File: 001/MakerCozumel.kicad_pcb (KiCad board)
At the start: 2 copper layers, 60.3 x 54.2 mm, 5 parts

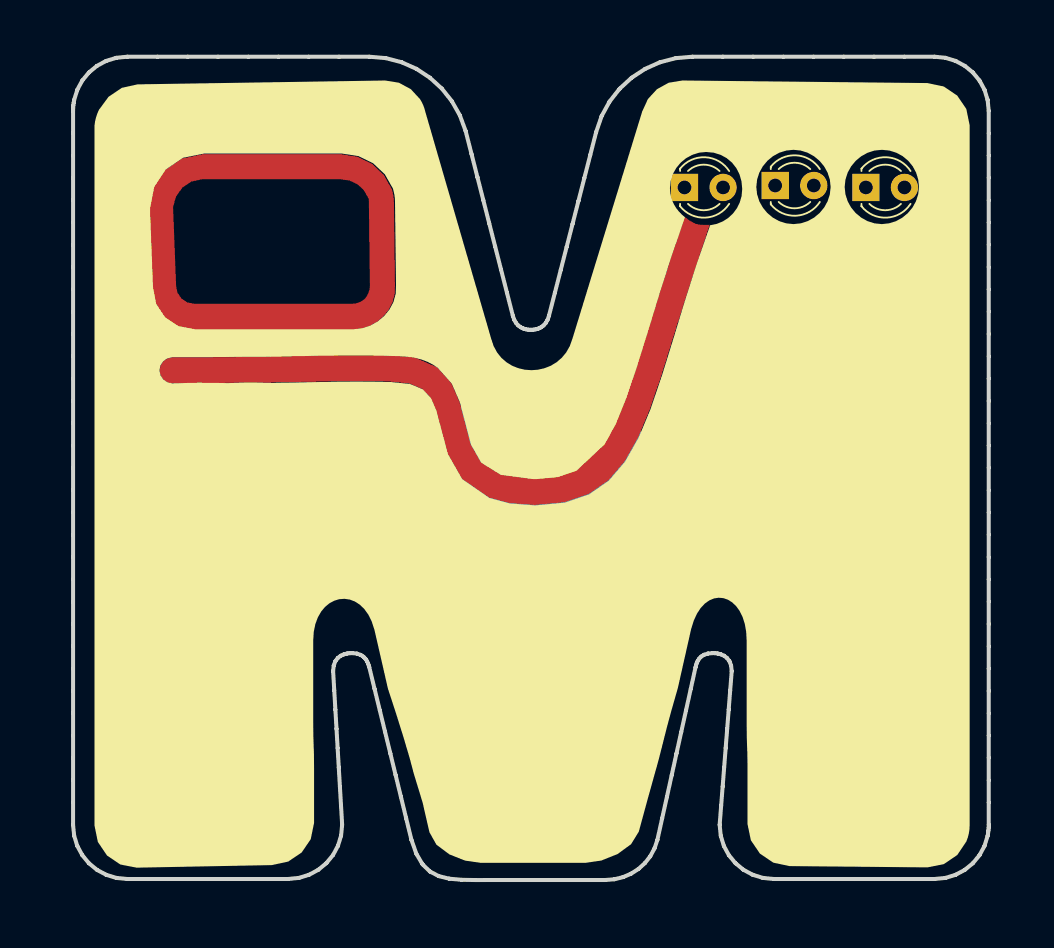
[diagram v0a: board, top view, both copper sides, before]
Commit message: Update 15 Nov 2018
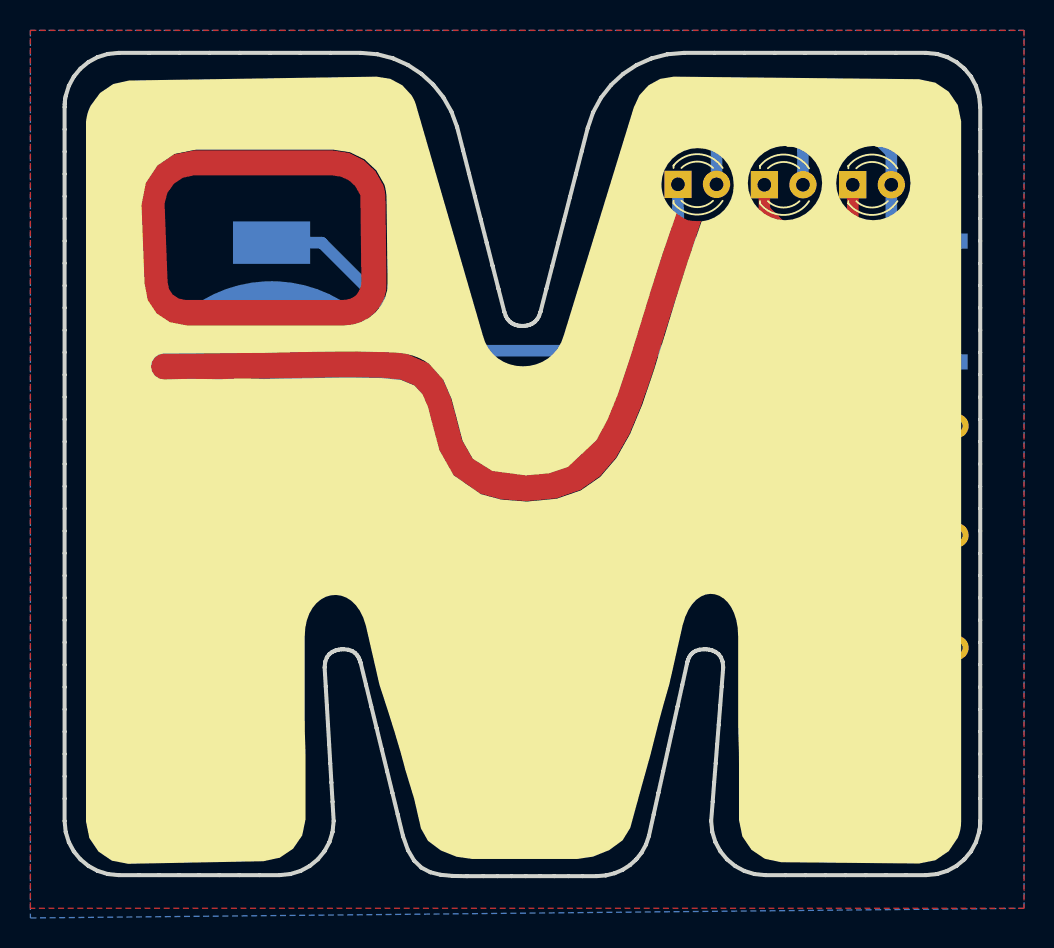
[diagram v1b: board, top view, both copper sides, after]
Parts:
- removed CR2032_MPD_BK912_SMT: VAL**, Battery:CR2032_MPD_BK912_SMT
- removed REF** (x3): LED_D3.0mm, LED_THT:LED_D3.0mm
- removed svg2mod: G***, Cozumel:Ment.All.01
- added BT1: Battery_Cell, Battery:CR2032_MPD_BK912_SMT, B.Cu at (121.9, 101.6)
- added D1: LED, LED_THT:LED_D3.0mm, F.Cu at (148.7, 86.3)
- added D2: LED, LED_THT:LED_D3.0mm, F.Cu at (154.4, 86.4)
- added D3: LED, LED_THT:LED_D3.0mm, F.Cu at (160.2, 86.4)
- added P1: Edge, Cozumel:Ment.All.01, F.Cu at (138.4, 104.8)
- added R1: R, Resistor_THT:R_Axial_DIN0309_L9.0mm_D3.2mm_P12.70mm_Horizontal, B.Cu at (154.3, 102.2)
- added R2: R, Resistor_THT:R_Axial_DIN0309_L9.0mm_D3.2mm_P12.70mm_Horizontal, B.Cu at (154.3, 109.4)
- added R3: R, Resistor_THT:R_Axial_DIN0309_L9.0mm_D3.2mm_P12.70mm_Horizontal, B.Cu at (154.3, 116.8)
- added SW1: SW_SPDT, HG:MSK12C02, B.Cu at (167.6, 90.2)
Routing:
- net Net-(BT1-Pad1): track 0.00 -> 46.5 mm
- net Net-(D3-Pad1): track 0.00 -> 38.2 mm
- net Net-(D2-Pad1): track 0.00 -> 31.2 mm
- net Net-(D1-Pad2): track 0.00 -> 26.2 mm
- net Net-(D1-Pad1): track 0.00 -> 18.2 mm, vias 0 -> 1
- net GND: vias 0 -> 1
- added copper zone on B.Cu, net GND
- added copper zone on F.Cu, net GND
